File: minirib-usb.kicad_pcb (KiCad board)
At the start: 2 copper layers, 49.5 x 22.5 mm, 54 parts, among them J1 USB_B_Micro, J2 SB9600 Out, Q1 MMST3904-7-F, Q2 MMST3906-7-F, Q3 MMST3906-7-F, Q4 MMST3904-7-F, Q5 MMST3904-7-F, Q6 MMST3904-7-F, Q7 MMST3904-7-F, Q8 MMST3906-7-F, Q9 MMST3906-7-F, U1 CH340G, U2 MCP6491T-E, Y1 12MHz

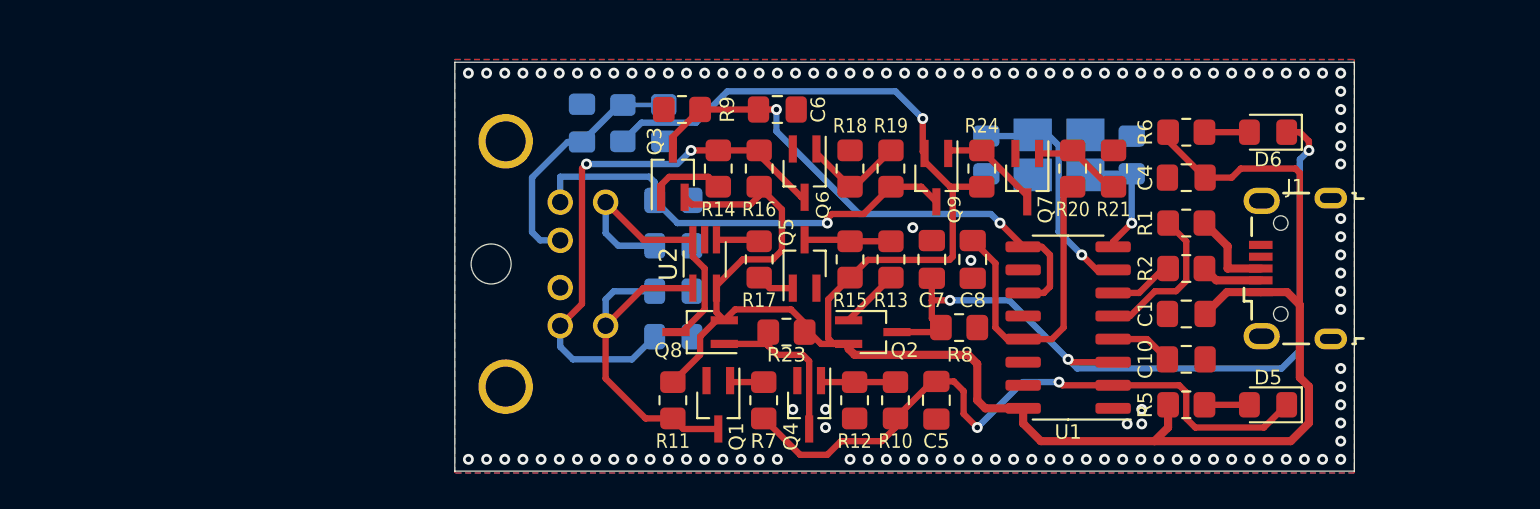
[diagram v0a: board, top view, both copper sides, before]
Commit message: finalized schematic and pcb
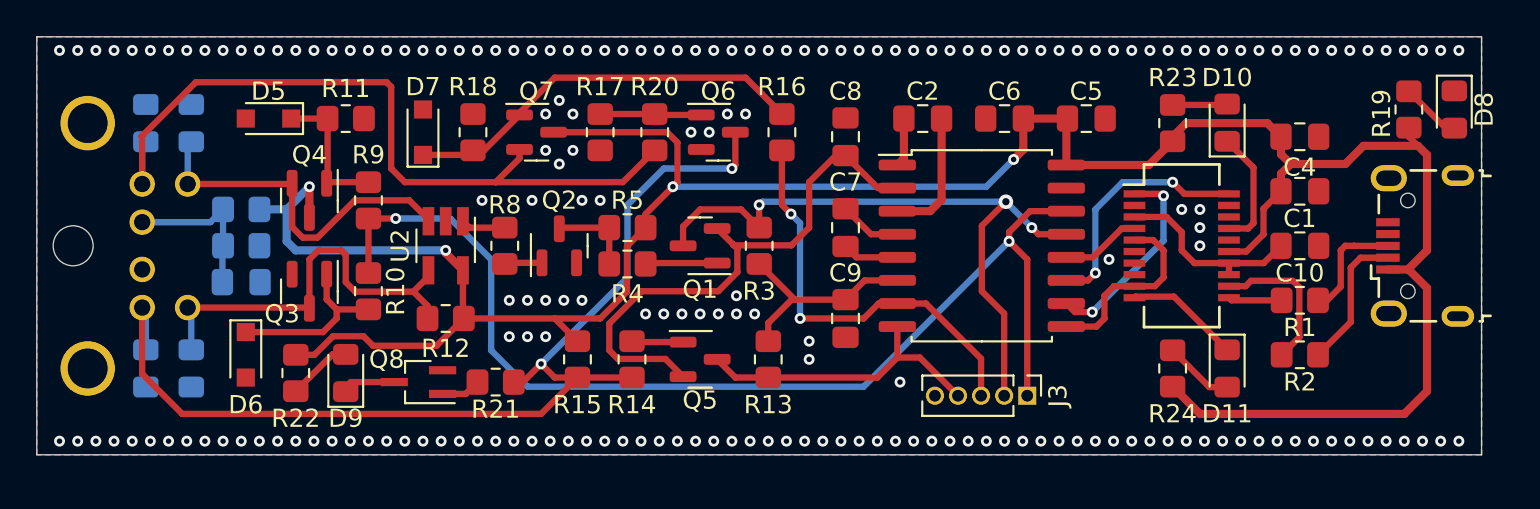
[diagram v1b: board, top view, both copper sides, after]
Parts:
- removed G***: LOGO, w3axl-logos:logo-4.2x4.2
- removed Q9: MMST3906-7-F, Package_TO_SOT_SMD:SOT-323_SC-70_Handsoldering
- removed Y1: 12MHz, Crystal:Crystal_SMD_SeikoEpson_FA238-4Pin_3.2x2.5mm_HandSoldering
- added D10: TXD, Diode_SMD:D_0805_2012Metric_Pad1.15x1.40mm_HandSolder, F.Cu at (165.5, 93.2)
- added D11: RXD, Diode_SMD:D_0805_2012Metric_Pad1.15x1.40mm_HandSolder, F.Cu at (165.5, 106.8)
- added D7: 1N4148, Diode_SMD:D_SOD-323_HandSoldering, F.Cu at (121.2, 93.8)
- added D8: PWR, Diode_SMD:D_0805_2012Metric_Pad1.15x1.40mm_HandSolder, F.Cu at (178.0, 92.5)
- added D9: BUSY, Diode_SMD:D_0805_2012Metric_Pad1.15x1.40mm_HandSolder, F.Cu at (117.0, 107.0)
- added J3: RS232, Connector_PinHeader_1.27mm:PinHeader_1x05_P1.27mm_Vertical, F.Cu at (154.5, 108.2)
- added R22: 1k5, Resistor_SMD:R_0805_2012Metric_Pad1.20x1.40mm_HandSolder, F.Cu at (114.2, 107.0)
- added U3: MAX232, Package_SO:SOIC-16W_7.5x10.3mm_P1.27mm, F.Cu at (152.0, 100.0)
- C2, C9: value 22pF -> 1uF; moved to F.Cu
- C5: value 220pF -> 0.1uF
- C6, C7, C8: value 220pF -> 1uF
- D5: value TXLED -> 1N4148; footprint Diode_SMD:D_0805_2012Metric_Pad1.15x1.40mm_HandSolder -> Diode_SMD:D_SOD-323_HandSoldering
- D6: value RXLED -> 1N4148; footprint Diode_SMD:D_0805_2012Metric_Pad1.15x1.40mm_HandSolder -> Diode_SMD:D_SOD-323_HandSoldering
- J2: value SB9600 Out -> Mini-DIN-6-Shielded
- Q1, Q5: value MMST3904-7-F -> MMBT3906; footprint Package_TO_SOT_SMD:SOT-323_SC-70_Handsoldering -> Package_TO_SOT_SMD:SOT-23
- Q2, Q3: value MMST3906-7-F -> MMBT3904; footprint Package_TO_SOT_SMD:SOT-323_SC-70_Handsoldering -> Package_TO_SOT_SMD:SOT-23
- Q4, Q6, Q7: value MMST3904-7-F -> MMBT3904; footprint Package_TO_SOT_SMD:SOT-323_SC-70_Handsoldering -> Package_TO_SOT_SMD:SOT-23
- Q8: value MMST3906-7-F -> BSS138W
- R10: value 4k7 -> 9k1
- R11: value 4k7 -> 47k
- R12: value 20k -> 10k
- R13, R19, R23, R24: value 4k7 -> 1k5
- R14, R15, R20: value 4k7 -> 10k
- R18: value 4k7 -> 20k
- R21: value 20k -> 1k5
- R3: value 3k -> 1k5; moved to F.Cu
- R4: value 1k5 -> 10k; moved to F.Cu
- R5: value 1k5 -> 10k
- R6: value 1k5 -> 39k; moved to B.Cu
- R7: value 4k7 -> 10k; moved to B.Cu
- R8: value 2k2 -> 20k
- R9: value 2k2 -> 9k1
- U1: value CH340G -> FT231XS; footprint Package_SO:SOIC-16_3.9x9.9mm_P1.27mm -> Package_SO:SSOP-20_3.9x8.7mm_P0.635mm
- U2: value MCP6491T-E -> TL071; footprint Package_TO_SOT_SMD:SOT-353_SC-70-5_Handsoldering -> Package_TO_SOT_SMD:SOT-23-5_HandSoldering
- moved D6 57.6 mm to (111.5, 106.0), turned to -90 degrees
- moved D5 57.2 mm to (112.8, 93.0)
- moved R6 52.2 mm to (111.2, 98.0)
- moved R21 36.0 mm to (125.2, 107.5), turned to 0 degrees
- moved R5 32.3 mm to (132.5, 99.0), turned to 180 degrees
- moved R7 30.0 mm to (111.2, 100.0), turned to 0 degrees
- moved Q4 29.7 mm to (115.0, 97.5)
- moved R10 29.6 mm to (118.2, 102.5), turned to 90 degrees
- moved D2 29.3 mm to (106.0, 93.2), turned to 90 degrees
- moved D3 29.1 mm to (106.0, 106.8), turned to -90 degrees
- moved R19 28.7 mm to (175.5, 92.5), turned to -90 degrees
- moved D1 27.4 mm to (108.5, 93.2), turned to 90 degrees
- moved Q7 27.1 mm to (127.5, 93.8), turned to 0 degrees
- moved D4 26.9 mm to (108.5, 106.8), turned to -90 degrees
- moved R8 25.4 mm to (125.8, 100.0), turned to -90 degrees
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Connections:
- C2 pad 2: GND -> Net-(C2-Pad2)
- C5 pad 1: TXD -> +5V
- C6 pad 1: ~{CTS} -> +5V
- C7 pad 1: RXD -> Net-(C7-Pad1)
- C7 pad 2: GND -> Net-(C7-Pad2)
- C8 pad 1: ~{DTR} -> +8V
- C9 pad 1: Net-(C9-Pad1) -> GND
- C9 pad 2: GND -> -8V
- D5 pad 1: TXD -> Net-(D5-Pad1)
- D5 pad 2: Net-(D5-Pad2) -> GND
- D6 pad 1: RXD -> Net-(D6-Pad1)
- D6 pad 2: Net-(D6-Pad2) -> GND
- Q1 pad 2: GND -> +8V
- Q1 pad 3: BUS+ -> RXD
- Q2 pad 2: +5V -> GND
- Q2 pad 3: RXD -> Net-(Q2-Pad3)
- Q3 pad 1: Net-(Q3-Pad1) -> Net-(D6-Pad1)
- Q3 pad 2: +5V -> GND
- Q3 pad 3: ~{CTS} -> BUS+
- Q4 pad 1: Net-(Q4-Pad1) -> Net-(D5-Pad1)
- Q4 pad 2: GND -> BUS-
- Q4 pad 3: Net-(Q4-Pad3) -> +5V
- Q5 pad 2: GND -> +8V
- Q5 pad 3: Net-(Q5-Pad3) -> CTS
- Q7 pad 1: Net-(Q7-Pad1) -> Net-(D7-Pad1)
- Q7 pad 2: GND -> ~{BUSY}
- Q7 pad 3: Net-(Q7-Pad3) -> +5V
- Q8 pad 1: Net-(Q4-Pad3) -> Net-(Q8-Pad1)
- Q8 pad 2: +5V -> GND
- Q8 pad 3: BUS- -> Net-(D9-Pad1)
- R10 pad 1: Net-(Q4-Pad1) -> Net-(D6-Pad1)
- R11 pad 1: BUS+ -> Net-(D5-Pad1)
- R11 pad 2: +5V -> GND
- R12 pad 1: GND -> +5V
- R12 pad 2: Net-(Q4-Pad1) -> BUS+
- R13 pad 1: Net-(Q5-Pad3) -> CTS
- R13 pad 2: Net-(Q2-Pad1) -> -8V
- R14 pad 1: Net-(Q3-Pad1) -> BUSY
- R14 pad 2: BUSY -> Net-(Q5-Pad1)
- R15 pad 1: Net-(Q5-Pad3) -> BUSY
- R16 pad 1: BUSY -> Net-(D7-Pad1)
- R16 pad 2: +5V -> DTR
- R17 pad 1: Net-(Q5-Pad1) -> Net-(Q6-Pad1)
- R17 pad 2: Net-(R17-Pad2) -> GND
- R18 pad 1: GND -> Net-(D7-Pad1)
- R18 pad 2: Net-(Q6-Pad1) -> GND
- R19 pad 1: ~{BUSY} -> Net-(D8-Pad2)
- R19 pad 2: Net-(Q6-Pad1) -> +5V
- R20 pad 1: Net-(Q7-Pad1) -> ~{BUSY}
- R20 pad 2: ~{DTR} -> Net-(Q6-Pad1)
- R21 pad 1: GND -> Net-(Q8-Pad1)
- R21 pad 2: Net-(Q7-Pad1) -> BUSY
- R23 pad 1: Net-(Q4-Pad3) -> Net-(D10-Pad2)
- R24 pad 1: Net-(Q7-Pad3) -> Net-(D11-Pad2)
- R3 pad 1: BIAS -> RXD
- R3 pad 2: +5V -> -8V
- R4 pad 1: GND -> Net-(Q1-Pad1)
- R4 pad 2: BIAS -> Net-(Q2-Pad3)
- R5 pad 2: Net-(D5-Pad2) -> Net-(Q2-Pad3)
- R6 pad 1: Net-(D6-Pad2) -> +5V
- R6 pad 2: +5V -> BIAS
- R7 pad 1: Net-(Q1-Pad1) -> BIAS
- R7 pad 2: TXD -> GND
- R8 pad 1: GND -> Net-(R8-Pad1)
- R8 pad 2: RXD -> Net-(Q2-Pad1)
- R9 pad 1: GND -> Net-(D5-Pad1)
- R9 pad 2: ~{CTS} -> TXD
- U1 pad 1: GND -> ~{DTR_TTL}
- U1 pad 10: unconnected-(U1-Pad10) -> ~{RXLED}
- U1 pad 11: ~{CTS} -> Net-(R1-Pad1)
- U1 pad 12: unconnected-(U1-Pad12) -> Net-(R2-Pad2)
- U1 pad 13: ~{DTR} -> Net-(C10-Pad1)
- U1 pad 14: unconnected-(U1-Pad14) -> Net-(C10-Pad1)
- U1 pad 15: unconnected-(U1-Pad15) -> +5V
- U1 pad 16: +5V -> GND
- U1 pad 2: TXD -> unconnected-(U1-Pad2)
- U1 pad 3: RXD -> Net-(C10-Pad1)
- U1 pad 4: Net-(C10-Pad1) -> RXD_TTL
- U1 pad 5: Net-(R1-Pad1) -> ~{CTS_TTL}
- U1 pad 6: Net-(R2-Pad2) -> GND
- U1 pad 7: Net-(C2-Pad1) -> unconnected-(U1-Pad7)
- U1 pad 8: Net-(C9-Pad1) -> unconnected-(U1-Pad8)
- U1 pad 9: ~{CTS} -> ~{CTS_TTL}
- U2 pad 1: Net-(R17-Pad2) -> Net-(R8-Pad1)
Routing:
- net +8V: track 0.00 -> 30.5 mm
- net ~{CTS}: track 29.4 -> 0.00 mm, vias 2 -> 0
- net BUSY: track 30.2 -> 58.3 mm
- net TXD: track 36.8 -> 61.4 mm
- net DTR: track 0.00 -> 23.3 mm, vias 0 -> 2
- net Net-(D7-Pad1): track 0.00 -> 22.4 mm
- net +5V: track 128.2 -> 146.1 mm, vias 1 -> 4
- net ~{DTR}: track 17.5 -> 0.00 mm
- net ~{BUSY}: track 25.1 -> 42.5 mm, vias 1 -> 0
- net CTS: track 0.00 -> 16.7 mm
- net TXD_TTL: track 0.00 -> 13.5 mm, vias 0 -> 2
- net -8V: track 0.00 -> 11.8 mm
- net ~{DTR_TTL}: track 0.00 -> 11.3 mm, vias 0 -> 2
- net ~{CTS_TTL}: track 0.00 -> 10.5 mm
- net Net-(C2-Pad1): track 12.9 -> 2.75 mm, vias 1 -> 0
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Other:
- board size 49.5 x 22.5 mm -> 79.5 x 23 mm
- board text removed: "MiniRIB USB rev B - 2022/01/04"
